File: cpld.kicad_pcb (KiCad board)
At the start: 2 copper layers, 30 parts, among them IC1 MCP1726-3302E_SN, IC2 EPM3064ATC44-7N, J1 USB_OTG, J2 INPUTS, J3 OUTPUTS, J4 Conn_ARM_JTAG_SWD_10, SW1 POWER_SW, SW2 SW_DIP_x01, SW3 SW_DIP_x01, SW4 SW_DIP_x01, SW5 SW_DIP_x01, Y1 ECS-2033-500-BN-TR3

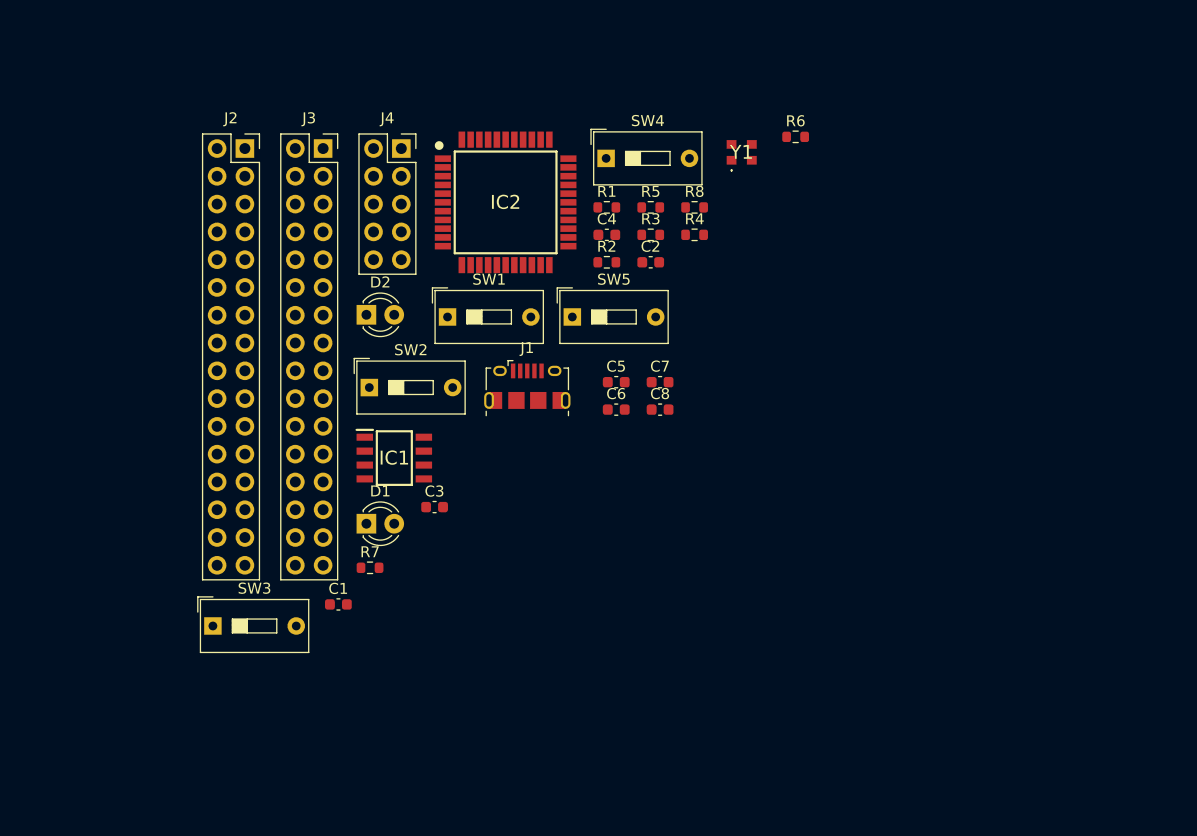
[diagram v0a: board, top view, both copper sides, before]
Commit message: Final PCB
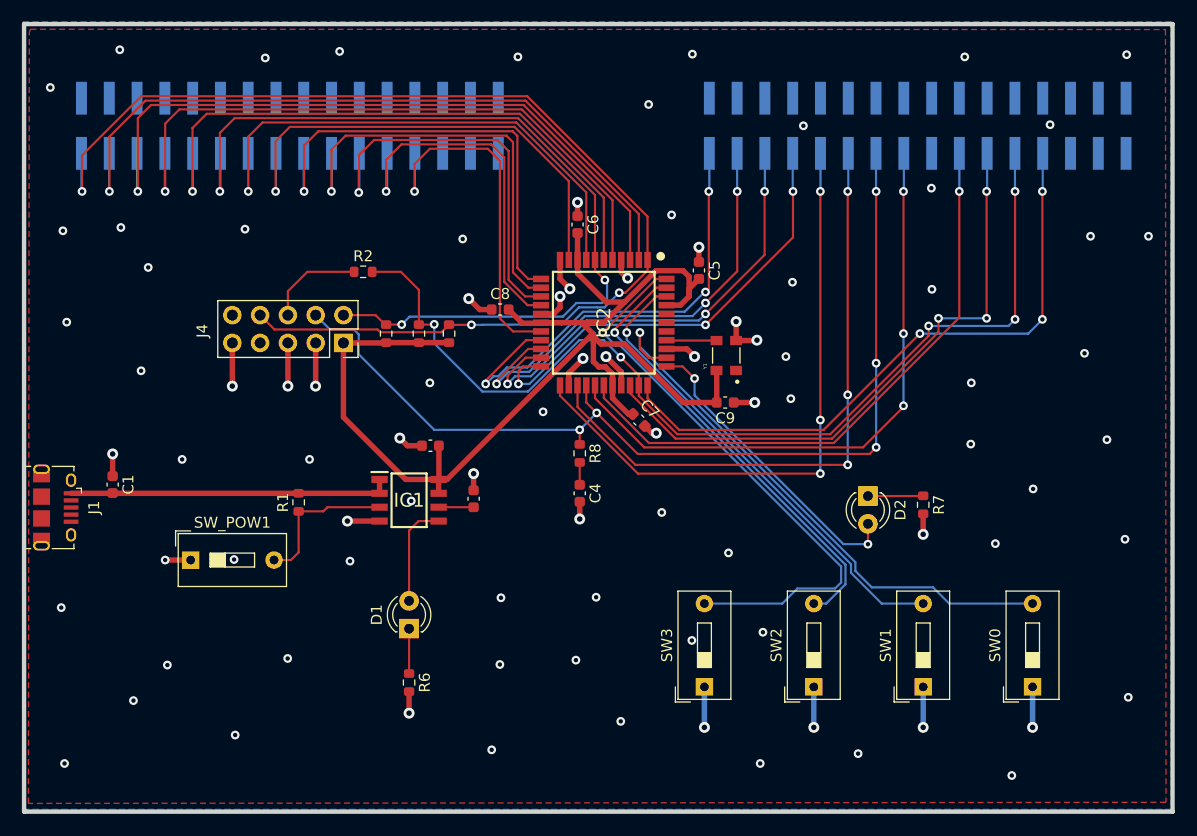
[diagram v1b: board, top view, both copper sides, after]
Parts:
- removed SW4, SW5: SW_DIP_x01, Button_Switch_THT:SW_DIP_SPSTx01_Slide_9.78x4.72mm_W7.62mm_P2.54mm
- added C9: 0.1u, Capacitor_SMD:C_0603_1608Metric, F.Cu at (152.2, 93.3)
- added SW0: SW_DIP_x01, Button_Switch_THT:SW_DIP_SPSTx01_Slide_9.78x4.72mm_W7.62mm_P2.54mm, F.Cu at (180.3, 119.3)
- added SW_POW1: POWER_SW, Button_Switch_THT:SW_DIP_SPSTx01_Slide_9.78x4.72mm_W7.62mm_P2.54mm, F.Cu at (103.3, 107.7)
- C2: value 1000p -> 1u
- J2, J3: footprint Connector_PinSocket_2.54mm:PinSocket_2x16_P2.54mm_Vertical -> Connector_PinSocket_2.54mm:PinSocket_2x16_P2.54mm_Vertical_SMD; moved to B.Cu
- SW1: value POWER_SW -> SW_DIP_x01
- Y1: value ECS-2033-500-BN-TR3 -> ECS-TXO-3225-250-TR; footprint ECS2033:ECS2033500BNTR3 -> ECS_3225:OSC_ECS-TXO-3225-250-TR
- moved R6 61.1 mm to (123.3, 118.9), turned to -90 degrees
- moved SW1 55.1 mm to (170.3, 119.3), turned to 90 degrees
- moved J3 54.4 mm to (169.8, 68.0), turned to -90 degrees
- moved R7 50.9 mm to (170.3, 102.7), turned to -90 degrees
- moved SW2 49.0 mm to (160.3, 119.3), turned to 90 degrees
- moved D2 48.8 mm to (165.2, 101.8), turned to -90 degrees
- moved SW3 45.3 mm to (150.3, 119.3), turned to 90 degrees
- moved J1 44.5 mm to (91.0, 102.9), turned to -90 degrees
- moved R1 39.0 mm to (113.2, 102.4), turned to 90 degrees
- moved C2 27.0 mm to (129.2, 102.1), turned to 90 degrees
- moved R4 26.8 mm to (124.2, 87.0), turned to 90 degrees
- moved R3 25.8 mm to (121.2, 87.0), turned to -90 degrees
- moved R8 24.8 mm to (138.9, 98.0), turned to -90 degrees
- moved C4 23.8 mm to (138.9, 101.6), turned to -90 degrees
- moved C1 23.4 mm to (96.2, 100.8), turned to -90 degrees
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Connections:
- D1 pad 1: GND -> Net-(D1-Pad1)
- D1 pad 2: Net-(D1-Pad2) -> /POWER_LED
- D2 pad 1: GND -> Net-(D2-Pad1)
- D2 pad 2: Net-(D2-Pad2) -> /STATUS_LED
- IC2 pad 1: /TDI -> /DI0/TDI
- IC2 pad 10: /DI5 -> /DI7
- IC2 pad 12: /DI6 -> /DI8
- IC2 pad 13: /DI7 -> /DI9
- IC2 pad 14: /DI8 -> /DI10
- IC2 pad 15: /DI9 -> /DI11
- IC2 pad 18: /DO0 -> /DI12
- IC2 pad 19: /DO1 -> /DO0
- IC2 pad 2: /DI0 -> /DI1
- IC2 pad 20: /DO2 -> /DO1
- IC2 pad 21: /DO3 -> /DO2
- IC2 pad 22: /DO4 -> /DO3
- IC2 pad 23: /DO5 -> /DO4
- IC2 pad 25: /DO6 -> /DO5
- IC2 pad 26: /TCK -> /DO6/TCK
- IC2 pad 28: /DO8 -> /DO9
- IC2 pad 3: /DI1 -> /DI2
- IC2 pad 31: /DO9 -> /DO10
- IC2 pad 32: /TDO -> /DO11/TDO
- IC2 pad 33: unconnected-(IC2-Pad33) -> /DO12
- IC2 pad 34: /SW_B0 -> /STATUS_LED
- IC2 pad 35: /SW_B1 -> /SW_B0
- IC2 pad 42: /SW_B2 -> /SW_B1
- IC2 pad 43: /SW_B3 -> /SW_B2
- IC2 pad 44: unconnected-(IC2-Pad44) -> /SW_B3
- IC2 pad 5: /DI2 -> /DI3
- IC2 pad 6: /DI3 -> /DI4
- IC2 pad 7: /TMS -> /DI5/TMS
- IC2 pad 8: /DI4 -> /DI6
- J2 pad 1: /DI0 -> /DI0/TDI
- J2 pad 10: /DI9 -> GND
- J2 pad 11: unconnected-(J2-Pad11) -> /DI5/TMS
- J2 pad 12: unconnected-(J2-Pad12) -> GND
- J2 pad 13: unconnected-(J2-Pad13) -> /DI6
- J2 pad 14: unconnected-(J2-Pad14) -> GND
- J2 pad 15: unconnected-(J2-Pad15) -> /DI7
- J2 pad 16: unconnected-(J2-Pad16) -> GND
- J2 pad 17: GND -> /DI8
- J2 pad 19: GND -> /DI9
- J2 pad 2: /DI1 -> GND
- J2 pad 21: GND -> /DI10
- J2 pad 23: GND -> /DI11
- J2 pad 25: GND -> /DI12
- J2 pad 27: GND -> unconnected-(J2-Pad27)
- J2 pad 29: GND -> unconnected-(J2-Pad29)
- J2 pad 3: /DI2 -> /DI1
- J2 pad 31: GND -> unconnected-(J2-Pad31)
- J2 pad 4: /DI3 -> GND
- J2 pad 5: /DI4 -> /DI2
- J2 pad 6: /DI5 -> GND
- J2 pad 7: /DI6 -> /DI3
- J2 pad 8: /DI7 -> GND
- J2 pad 9: /DI8 -> /DI4
- J3 pad 10: /DO9 -> GND
- J3 pad 11: unconnected-(J3-Pad11) -> /DO5
- J3 pad 12: unconnected-(J3-Pad12) -> GND
- J3 pad 13: unconnected-(J3-Pad13) -> /DO6/TCK
- J3 pad 14: unconnected-(J3-Pad14) -> GND
- J3 pad 15: unconnected-(J3-Pad15) -> /DO7
- J3 pad 16: unconnected-(J3-Pad16) -> GND
- J3 pad 17: GND -> /DO8
- J3 pad 19: GND -> /DO9
- J3 pad 2: /DO1 -> GND
- J3 pad 21: GND -> /DO10
- J3 pad 23: GND -> /DO11/TDO
- J3 pad 25: GND -> /DO12
- J3 pad 27: GND -> unconnected-(J3-Pad27)
- J3 pad 29: GND -> unconnected-(J3-Pad29)
- J3 pad 3: /DO2 -> /DO1
- J3 pad 31: GND -> unconnected-(J3-Pad31)
- J3 pad 4: /DO3 -> GND
- J3 pad 5: /DO4 -> /DO2
- J3 pad 6: /DO5 -> GND
- J3 pad 7: /DO6 -> /DO3
- J3 pad 8: /DO7 -> GND
- J3 pad 9: /DO8 -> /DO4
- J4 pad 2: /TMS -> /DI5/TMS
- J4 pad 4: /TCK -> /DO6/TCK
- J4 pad 8: /TDI -> /DI0/TDI
- R2 pad 2: /TDO -> /DO11/TDO
- R3 pad 1: /TMS -> /DI5/TMS
- R4 pad 2: /TDO -> /DO11/TDO
- R5 pad 2: /TDI -> /DI0/TDI
- R6 pad 1: /POWER_LED -> Net-(D1-Pad1)
- R6 pad 2: Net-(D1-Pad2) -> GND
- R7 pad 1: /STATUS_LED -> Net-(D2-Pad1)
- R7 pad 2: Net-(D2-Pad2) -> GND
- R8 pad 1: /TCK -> /DO6/TCK
- SW1 pad 2: Net-(IC1-Pad3) -> /SW_B1
- SW2 pad 2: /SW_B0 -> /SW_B2
- SW3 pad 2: /SW_B1 -> /SW_B3
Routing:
- net +3.3V: track 0.00 -> 112.3 mm
- net /DI0/TDI: track 0.00 -> 108.6 mm, vias 0 -> 3
- net /DO11/TDO: track 0.00 -> 93.1 mm, vias 0 -> 5
- net /DO6/TCK: track 0.00 -> 90.2 mm, vias 0 -> 5
- net /DI5/TMS: track 0.00 -> 82.0 mm, vias 0 -> 3
- net GND: track 0.00 -> 72.2 mm, vias 0 -> 88
- net /DI1: track 0.00 -> 66.7 mm, vias 0 -> 1
- net /DI2: track 0.00 -> 64.2 mm, vias 0 -> 1
- net /DI3: track 0.00 -> 60.0 mm, vias 0 -> 1
- net /DO12: track 0.00 -> 57.8 mm, vias 0 -> 3
- net /DO5: track 0.00 -> 57.4 mm, vias 0 -> 3
- net /DO4: track 0.00 -> 57.0 mm, vias 0 -> 3
- net /DI4: track 0.00 -> 56.3 mm, vias 0 -> 1
- net /DO7: track 0.00 -> 55.9 mm, vias 0 -> 3
- net /DO10: track 0.00 -> 55.4 mm, vias 0 -> 3
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- added copper zone on B.Cu, net GND
- added copper zone on F.Cu, net GND
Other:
- board outline added: 105 x 72 mm
